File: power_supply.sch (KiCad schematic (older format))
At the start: 5 parts, among them P0 CONN_4, U1 MAX660, U3 DMP2066LSD

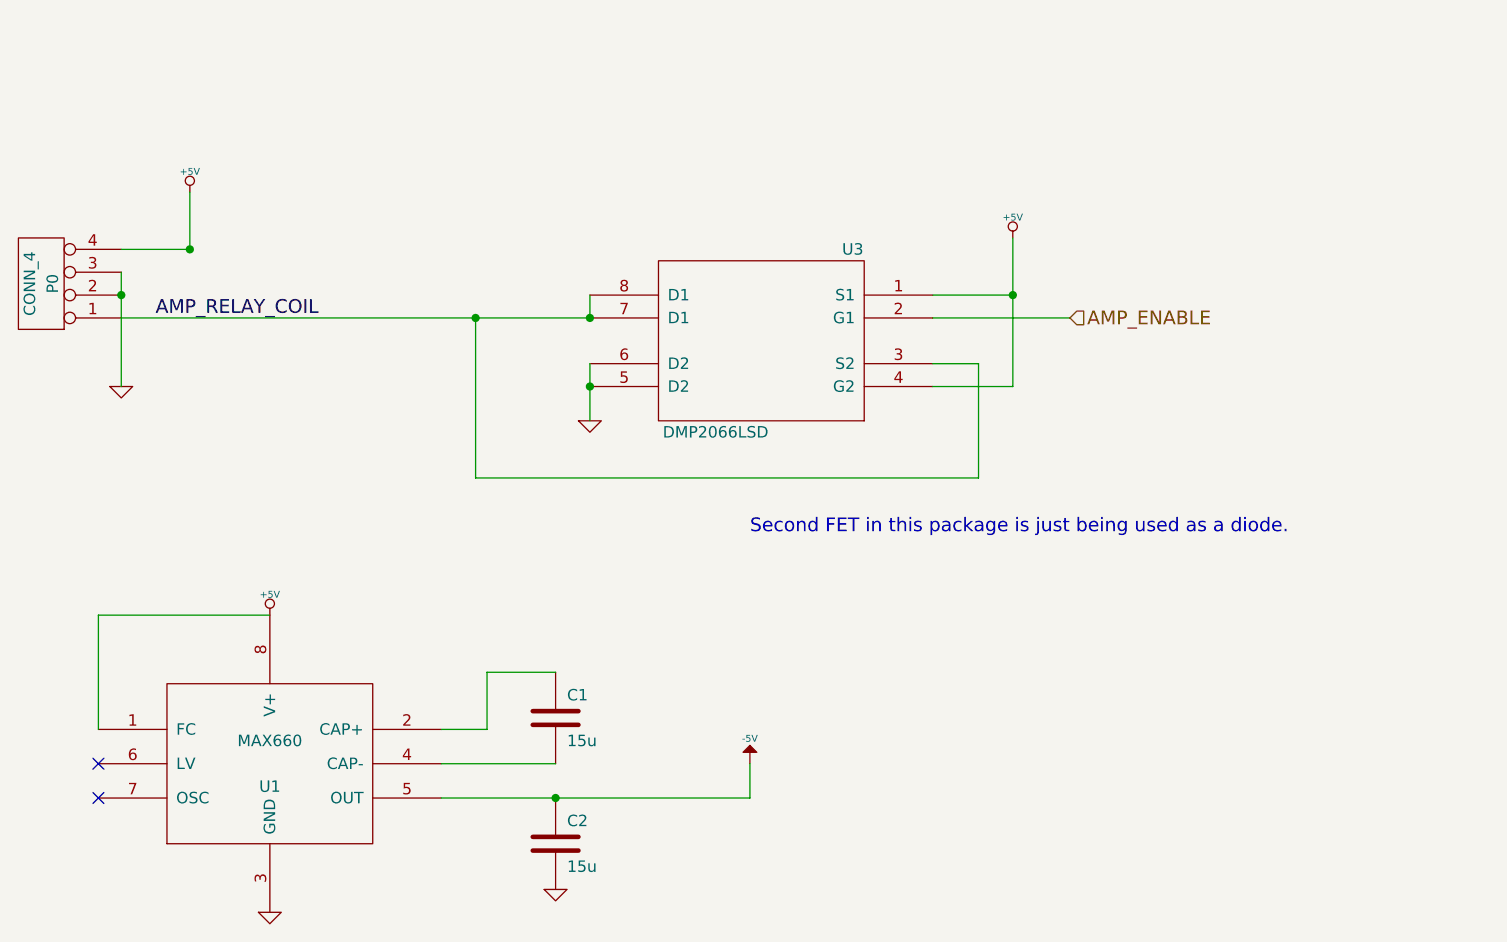
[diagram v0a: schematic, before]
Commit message: Final board as sent for fab.
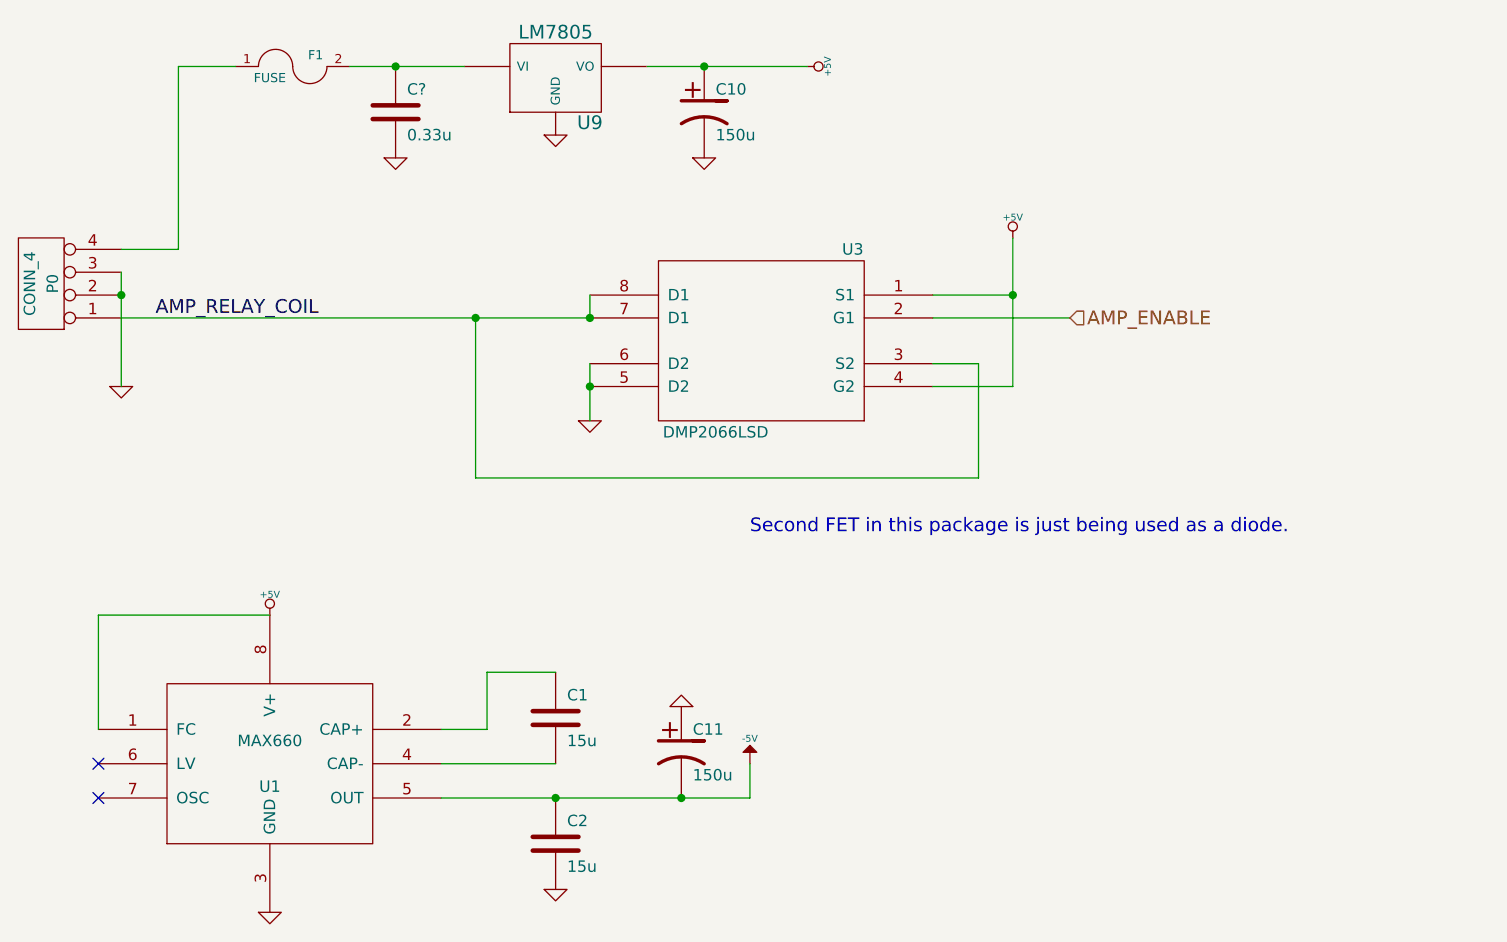
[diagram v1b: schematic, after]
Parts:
- added C10, C11: 150u, symbol CP1
- added C?: 0.33u, symbol C
- added F1: FUSE, symbol FUSE
- added U9: LM7805, symbol LM7805
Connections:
- net +5V: now also C10.1, U9.VO; no longer P0.4 (P4)
- net -5V: now also C11.2
- net GND: now also C10.2, C11.1, C?.2, U9.GND
- new net: F1.1, P0.4 (P4)
- new net: C?.1, F1.2, U9.VI
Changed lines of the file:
@@
-EESchema Schematic File Version 2  date 8/1/2012 10:55:27 PM
+EESchema Schematic File Version 2  date 8/3/2012 1:01:40 PM
 LIBS:atmel
 LIBS:device
@@
 Sheet 3 3
 Title ""
-Date "2 aug 2012"
+Date "3 aug 2012"
 Rev ""
 Comp ""
@@
 Comment4 ""
 $EndDescr
+Connection ~ 4100 1900
+Wire Wire Line
+	3900 1900 4400 1900
+Wire Wire Line
+	3400 1900 3150 1900
+Wire Wire Line
+	3150 1900 3150 2700
+Wire Wire Line
+	3150 2700 2900 2700
+Connection ~ 4800 5100
+Wire Wire Line
+	5650 4950 5650 5100
+Wire Wire Line
+	5650 5100 4300 5100
+Wire Wire Line
+	4800 4550 4500 4550
+Wire Wire Line
+	4500 4550 4500 4800
+Wire Wire Line
+	4500 4800 4300 4800
+Connection ~ 4950 3300
+Wire Wire Line
+	4950 3200 4950 3450
+Wire Wire Line
+	6650 3200 6650 3700
+Wire Wire Line
+	6650 3200 6450 3200
+Connection ~ 6800 2900
+Wire Wire Line
+	6450 3000 7050 3000
+Connection ~ 4950 3000
+Wire Wire Line
+	2900 3300 2900 2800
+Wire Wire Line
+	2900 3000 4950 3000
+Connection ~ 2900 2900
+Wire Wire Line
+	6450 2900 6800 2900
+Wire Wire Line
+	4950 3000 4950 2900
+Wire Wire Line
+	6450 3300 6800 3300
+Wire Wire Line
+	6800 3300 6800 2650
+Wire Wire Line
+	4450 3000 4450 3700
+Connection ~ 4450 3000
+Wire Wire Line
+	4450 3700 6650 3700
+Wire Wire Line
+	4300 4950 4800 4950
+Wire Wire Line
+	2800 4800 2800 4300
+Wire Wire Line
+	2800 4300 3550 4300
+Connection ~ 5350 5100
+Wire Wire Line
+	5900 1900 5200 1900
+Connection ~ 5450 1900
+$Comp
+L GND #PWR?
+U 1 1 501C03E7
+P 4100 2300
+F 0 "#PWR?" H 4100 2300 30  0001 C CNN
+F 1 "GND" H 4100 2230 30  0001 C CNN
+	1    4100 2300
+	1    0    0    -1
+$EndComp
+$Comp
+L C C?
+U 1 1 501C03D0
+P 4100 2100
+F 0 "C?" H 4150 2200 50  0000 L CNN
+F 1 "0.33u" H 4150 2000 50  0000 L CNN
+	1    4100 2100
+	1    0    0    -1
+$EndComp
+$Comp
+L GND #PWR037
+U 1 1 501C00FA
+P 4800 2200
+F 0 "#PWR037" H 4800 2200 30  0001 C CNN
+F 1 "GND" H 4800 2130 30  0001 C CNN
+	1    4800 2200
+	1    0    0    -1
+$EndComp
+$Comp
+L LM7805 U9
+U 1 1 501C00DD
+P 4800 1950
+F 0 "U9" H 4950 1754 60  0000 C CNN
+F 1 "LM7805" H 4800 2150 60  0000 C CNN
+F 4 "497-2957-5-ND" H 4800 1950 60  0001 C CNN "Digikey"
+	1    4800 1950
+	1    0    0    -1
+$EndComp
+$Comp
+L GND #PWR038
+U 1 1 501BED49
+P 5350 4700
+F 0 "#PWR038" H 5350 4700 30  0001 C CNN
+F 1 "GND" H 5350 4630 30  0001 C CNN
+	1    5350 4700
+	-1   0    0    1
+$EndComp
+$Comp
+L GND #PWR039
+U 1 1 501BED47
+P 5450 2300
+F 0 "#PWR039" H 5450 2300 30  0001 C CNN
+F 1 "GND" H 5450 2230 30  0001 C CNN
+	1    5450 2300
+	1    0    0    -1
+$EndComp
+$Comp
+L CP1 C10
+U 1 1 501BED37
+P 5450 2100
+F 0 "C10" H 5500 2200 50  0000 L CNN
+F 1 "150u" H 5500 2000 50  0000 L CNN
+F 4 "P5138-ND" H 5450 2100 60  0001 C CNN "Digikey"
+	1    5450 2100
+	1    0    0    -1
+$EndComp
+$Comp
+L CP1 C11
+U 1 1 501BED26
+P 5350 4900
+F 0 "C11" H 5400 5000 50  0000 L CNN
+F 1 "150u" H 5400 4800 50  0000 L CNN
+F 4 "P5138-ND" H 5350 4900 60  0001 C CNN "Digikey"
+	1    5350 4900
+	1    0    0    -1
+$EndComp
+$Comp
+L FUSE F1
+U 1 1 501BEAB5
+P 3650 1900
+F 0 "F1" H 3750 1950 40  0000 C CNN
+F 1 "FUSE" H 3550 1850 40  0000 C CNN
+F 4 "507-1482-1-ND" H 3650 1900 60  0001 C CNN "Digikey"
+	1    3650 1900
+	1    0    0    -1
+$EndComp
 Text Notes 5650 3950 0    60   ~ 0
 Second FET in this package is just being used as a diode.
 NoConn ~ 2800 5100
-Wire Wire Line
-	3550 4300 2800 4300
-Wire Wire Line
-	2800 4300 2800 4800
-Wire Wire Line
-	4300 4950 4800 4950
-Wire Wire Line
-	4450 3700 6650 3700
-Connection ~ 4450 3000
-Wire Wire Line
-	4450 3700 4450 3000
-Wire Wire Line
-	6800 2650 6800 3300
-Wire Wire Line
-	6800 3300 6450 3300
-Wire Wire Line
-	4950 2900 4950 3000
-Wire Wire Line
-	6800 2900 6450 2900
-Connection ~ 2900 2900
-Connection ~ 3200 2700
-Wire Wire Line
-	4950 3000 2900 3000
-Wire Wire Line
-	2900 2800 2900 3300
-Wire Wire Line
-	3200 2450 3200 2700
-Connection ~ 4950 3000
-Wire Wire Line
-	6450 3000 7050 3000
-Wire Wire Line
-	3200 2700 2900 2700
-Connection ~ 6800 2900
-Wire Wire Line
-	6450 3200 6650 3200
-Wire Wire Line
-	6650 3200 6650 3700
-Wire Wire Line
-	4950 3450 4950 3200
-Connection ~ 4950 3300
-Wire Wire Line
-	4300 4800 4500 4800
-Wire Wire Line
-	4500 4800 4500 4550
-Wire Wire Line
-	4500 4550 4800 4550
-Wire Wire Line
-	4300 5100 5650 5100
-Wire Wire Line
-	5650 5100 5650 4950
-Connection ~ 4800 5100
 NoConn ~ 2800 4950
 $Comp
-L +5V #PWR033
+L +5V #PWR040
 U 1 1 5019EAE9
 P 3550 4300
-F 0 "#PWR033" H 3550 4390 20  0001 C CNN
+F 0 "#PWR040" H 3550 4390 20  0001 C CNN
 F 1 "+5V" H 3550 4390 30  0000 C CNN
 	1    3550 4300
@@
 $EndComp
 $Comp
-L GND #PWR034
+L GND #PWR041
 U 1 1 5019EADB
 P 3550 5600
-F 0 "#PWR034" H 3550 5600 30  0001 C CNN
+F 0 "#PWR041" H 3550 5600 30  0001 C CNN
 F 1 "GND" H 3550 5530 30  0001 C CNN
 	1    3550 5600
@@
 $EndComp
 $Comp
-L GND #PWR035
+L GND #PWR042
 U 1 1 5019EAD5
 P 4800 5500
-F 0 "#PWR035" H 4800 5500 30  0001 C CNN
+F 0 "#PWR042" H 4800 5500 30  0001 C CNN
 F 1 "GND" H 4800 5430 30  0001 C CNN
 	1    4800 5500
@@
 $EndComp
 $Comp
-L -5V #PWR036
+L -5V #PWR043
 U 1 1 5019EACF
 P 5650 4950
-F 0 "#PWR036" H 5650 5090 20  0001 C CNN
+F 0 "#PWR043" H 5650 5090 20  0001 C CNN
 F 1 "-5V" H 5650 5060 30  0000 C CNN
 	1    5650 4950
@@
 $EndComp
 $Comp
-L GND #PWR037
+L GND #PWR044
 U 1 1 50195E98
 P 4950 3450
-F 0 "#PWR037" H 4950 3450 30  0001 C CNN
+F 0 "#PWR044" H 4950 3450 30  0001 C CNN
 F 1 "GND" H 4950 3380 30  0001 C CNN
 	1    4950 3450
@@
 $EndComp
 $Comp
-L +5V #PWR038
+L +5V #PWR045
 U 1 1 50189DC4
 P 6800 2650
-F 0 "#PWR038" H 6800 2740 20  0001 C CNN
+F 0 "#PWR045" H 6800 2740 20  0001 C CNN
 F 1 "+5V" H 6800 2740 30  0000 C CNN
 	1    6800 2650
@@
 $EndComp
 $Comp
-L +5V #PWR039
+L +5V #PWR046
 U 1 1 50189DBE
-P 3200 2450
-F 0 "#PWR039" H 3200 2540 20  0001 C CNN
-F 1 "+5V" H 3200 2540 30  0000 C CNN
-	1    3200 2450
-	1    0    0    -1
+P 5900 1900
+F 0 "#PWR046" H 5900 1990 20  0001 C CNN
+F 1 "+5V" H 5900 1990 30  0000 C CNN
+	1    5900 1900
+	0    1    1    0
 $EndComp
 $Comp
@@
 AMP_RELAY_COIL
 $Comp
-L GND #PWR040
+L GND #PWR047
 U 1 1 50078FA5
 P 2900 3300
-F 0 "#PWR040" H 2900 3300 30  0001 C CNN
+F 0 "#PWR047" H 2900 3300 30  0001 C CNN
 F 1 "GND" H 2900 3230 30  0001 C CNN
 	1    2900 3300
